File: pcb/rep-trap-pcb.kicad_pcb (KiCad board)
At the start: 4 copper layers, 161 x 23 mm, 80 parts, among them J1 BATT+, J2 GND, J3 USB4105-GF-A, J4 VBUS, J5 SJ2-25773B-SMT-TR, J6 S2B-PH-K/DNP, J7 GND, SW1 SKRKAEE020, U1 AP2112K-3.3, U10 W25Q128JVS, U2 MCP73831/OT, U3 VL53L4CDV0DH/1, U4 VL53L4CDV0DH/1, U5 VL53L4CDV0DH/1, U6 VL53L4CDV0DH/1, U7 450405020524, U8 RP2040, Y3 ABMM2-12.000MHZ-E2-T

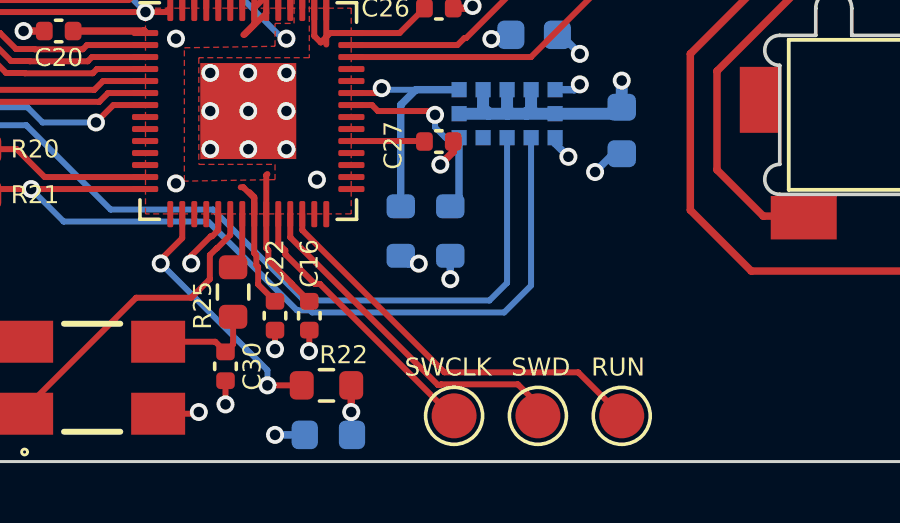
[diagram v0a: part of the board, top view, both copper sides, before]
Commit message: Added notes and ToDos to be worked on for REV.02
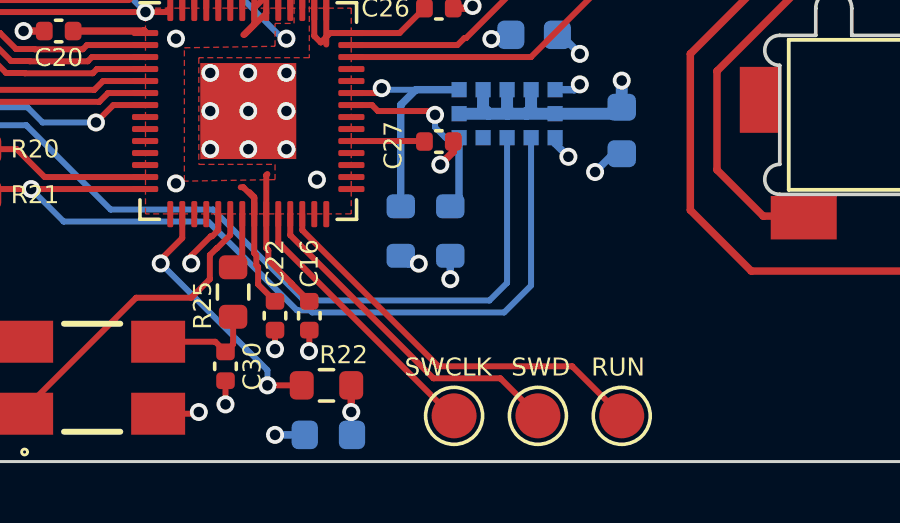
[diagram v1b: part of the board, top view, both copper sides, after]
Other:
- board text added: "- all connectors on one side (USB, Klinke) - exchange 18650 Battery Holder crap - apply heatsink guidelines to charger IC - number sensors"
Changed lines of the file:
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@@
     (effects (font (size 0.6 0.6) (thickness 0.15)) (justify left bottom))
+  )
+  (gr_text "- all connectors on one side (USB, Klinke)\n- exchange 18650 Battery Holder crap\n- apply heatsink guidelines to charger IC\n- number sensors " (at 111.887 125.603) (layer "Dwgs.User")
+    (effects (font (size 3 3) (thickness 0.3) bold) (justify left bottom))
   )
   (dimension (type aligned) (layer "F.Cu")
     (pts (xy 230.124 79.248) (xy 69.215 79.248))
     (height 11.7856)
-    (gr_text "160,9090 mm" (at 149.6695 65.6624) (layer "F.Cu")
+    (gr_text "160.9090 mm" (at 149.6695 65.6624) (layer "F.Cu")
       (effects (font (size 1.5 1.5) (thickness 0.3)))
     )
@@
     (pts (xy 230.124 102.235) (xy 230.124 79.248))
     (height 14.0208)
-    (gr_text "22,9870 mm" (at 242.3448 90.7415 90) (layer "F.Cu")
+    (gr_text "22.9870 mm" (at 242.3448 90.7415 90) (layer "F.Cu")
       (effects (font (size 1.5 1.5) (thickness 0.3)))
     )
@@
   (via (at 82.677 86.614) (size 0.6) (drill 0.35) (layers "F.Cu" "B.Cu") (net 4))
   (segment (start 191.855 100.641) (end 193.253 100.641) (width 0.2) (layer "F.Cu") (net 5))
+  (segment (start 199.617746 95.124503) (end 199.60439 95.124503) (width 0.2) (layer "F.Cu") (net 5))
+  (segment (start 199.377 96.152) (end 198.755 96.774) (width 0.2) (layer "F.Cu") (net 5))
+  (segment (start 191.135 99.921) (end 191.855 100.641) (width 0.2) (layer "F.Cu") (net 5))
+  (segment (start 198.755 96.774) (end 196.92 96.774) (width 0.2) (layer "F.Cu") (net 5))
+  (segment (start 199.377 95.351893) (end 199.377 96.152) (width 0.2) (layer "F.Cu") (net 5))
+  (segment (start 193.253 100.441) (end 193.253 100.641) (width 0.2) (layer "F.Cu") (net 5))
+  (segment (start 200.057 94.685249) (end 199.617746 95.124503) (width 0.2) (layer "F.Cu") (net 5))
+  (segment (start 196.92 96.774) (end 193.253 100.441) (width 0.2) (layer "F.Cu") (net 5))
+  (segment (start 200.057 93.9885) (end 200.057 94.685249) (width 0.2) (layer "F.Cu") (net 5))
   (segment (start 199.60439 95.124503) (end 199.377 95.351893) (width 0.2) (layer "F.Cu") (net 5))
-  (segment (start 196.92 96.774) (end 193.253 100.441) (width 0.2) (layer "F.Cu") (net 5))
-  (segment (start 191.135 99.921) (end 191.855 100.641) (width 0.2) (layer "F.Cu") (net 5))
-  (segment (start 200.057 94.685249) (end 199.617746 95.124503) (width 0.2) (layer "F.Cu") (net 5))
-  (segment (start 193.253 100.441) (end 193.253 100.641) (width 0.2) (layer "F.Cu") (net 5))
-  (segment (start 199.377 96.152) (end 198.755 96.774) (width 0.2) (layer "F.Cu") (net 5))
-  (segment (start 200.057 93.9885) (end 200.057 94.685249) (width 0.2) (layer "F.Cu") (net 5))
-  (segment (start 198.755 96.774) (end 196.92 96.774) (width 0.2) (layer "F.Cu") (net 5))
-  (segment (start 199.617746 95.124503) (end 199.60439 95.124503) (width 0.2) (layer "F.Cu") (net 5))
-  (segment (start 199.377 95.351893) (end 199.377 96.152) (width 0.2) (layer "F.Cu") (net 5))
   (segment (start 200.152 98.326) (end 199.898 98.58) (width 0.2) (layer "F.Cu") (net 6))
   (segment (start 200.152 97.409) (end 200.152 98.326) (width 0.2) (layer "F.Cu") (net 6))
@@
   (segment (start 204.0945 88.751) (end 210.08 88.751) (width 0.2) (layer "F.Cu") (net 50))
   (segment (start 210.08 88.751) (end 212.345 86.486) (width 0.2) (layer "F.Cu") (net 50))
-  (segment (start 203.044254 96.3135) (end 207.441754 100.711) (width 0.2) (layer "F.Cu") (net 51))
+  (segment (start 201.657 93.9885) (end 201.657 94.926246) (width 0.2) (layer "F.Cu") (net 51))
   (segment (start 207.441754 100.711) (end 207.518 100.711) (width 0.2) (layer "F.Cu") (net 51))
-  (segment (start 201.657 94.96396) (end 201.892998 95.199958) (width 0.2) (layer "F.Cu") (net 51))
-  (segment (start 201.892998 95.326958) (end 202.87954 96.3135) (width 0.2) (layer "F.Cu") (net 51))
-  (segment (start 202.87954 96.3135) (end 203.044254 96.3135) (width 0.2) (layer "F.Cu") (net 51))
-  (segment (start 201.657 93.9885) (end 201.657 94.96396) (width 0.2) (layer "F.Cu") (net 51))
-  (segment (start 201.892998 95.199958) (end 201.892998 95.326958) (width 0.2) (layer "F.Cu") (net 51))
-  (segment (start 207.083075 99.661) (end 209.643 99.661) (width 0.2) (layer "F.Cu") (net 52))
-  (segment (start 207.05756 99.686515) (end 207.083075 99.661) (width 0.2) (layer "F.Cu") (net 52))
-  (segment (start 210.312 100.33) (end 210.312 100.711) (width 0.2) (layer "F.Cu") (net 52))
-  (segment (start 206.982249 99.686515) (end 207.05756 99.686515) (width 0.2) (layer "F.Cu") (net 52))
-  (segment (start 202.057 94.761266) (end 206.982249 99.686515) (width 0.2) (layer "F.Cu") (net 52))
-  (segment (start 209.643 99.661) (end 210.312 100.33) (width 0.2) (layer "F.Cu") (net 52))
-  (segment (start 202.057 93.9885) (end 202.057 94.761266) (width 0.2) (layer "F.Cu") (net 52))
+  (segment (start 201.657 94.926246) (end 207.441754 100.711) (width 0.2) (layer "F.Cu") (net 51))
+  (segment (start 209.061 99.46) (end 210.312 100.711) (width 0.2) (layer "F.Cu") (net 52))
+  (segment (start 202.057 94.686661) (end 206.83034 99.46) (width 0.2) (layer "F.Cu") (net 52))
+  (segment (start 206.83034 99.46) (end 209.061 99.46) (width 0.2) (layer "F.Cu") (net 52))
+  (segment (start 202.057 93.9885) (end 202.057 94.686661) (width 0.2) (layer "F.Cu") (net 52))
   (segment (start 198.251975 86.376) (end 198.456839 86.580864) (width 0.2) (layer "F.Cu") (net 56))
   (segment (start 189.611 83.312) (end 191.77 85.471) (width 0.2) (layer "F.Cu") (net 56))
@@
   (segment (start 195.58 83.312) (end 197.044998 84.776998) (width 0.2) (layer "F.Cu") (net 60))
   (segment (start 197.044998 84.776998) (end 198.91501 84.776998) (width 0.2) (layer "F.Cu") (net 60))
-  (segment (start 202.457 94.520975) (end 207.197524 99.261499) (width 0.2) (layer "F.Cu") (net 66))
-  (segment (start 207.197524 99.261499) (end 211.656499 99.261499) (width 0.2) (layer "F.Cu") (net 66))
-  (segment (start 211.656499 99.261499) (end 213.106 100.711) (width 0.2) (layer "F.Cu") (net 66))
+  (segment (start 211.455 99.06) (end 213.106 100.711) (width 0.2) (layer "F.Cu") (net 66))
+  (segment (start 202.457 94.520975) (end 206.996025 99.06) (width 0.2) (layer "F.Cu") (net 66))
+  (segment (start 206.996025 99.06) (end 211.455 99.06) (width 0.2) (layer "F.Cu") (net 66))
   (segment (start 202.457 93.9885) (end 202.457 94.520975) (width 0.2) (layer "F.Cu") (net 66))
   (zone (net 1) (net_name "+3.3V") (layer "F.Cu") (hatch edge 0.5)
